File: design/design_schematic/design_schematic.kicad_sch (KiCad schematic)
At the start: 157 parts, among them IC2 XC9148G50CER-G, IC3 nRF52833-QDAA-R7, IC4 74AHCT125PW,118, IC5 MCP23018T-E_SS, IC6 XC9291B33D1R-G, J1 USB_C_Receptacle_USB2.0_16P, J2 Battery Pos, J3 Battery Neg, J4 OLED_128x32, J5 0781271220, J6 Conn_01x04, U2 BQ24072RGT, U3 USB6B1, U4 BQ27441-G1, U5 PEC11L-4015F-S0015, U6 PEC11L-4015F-S0015, X1 32MHz

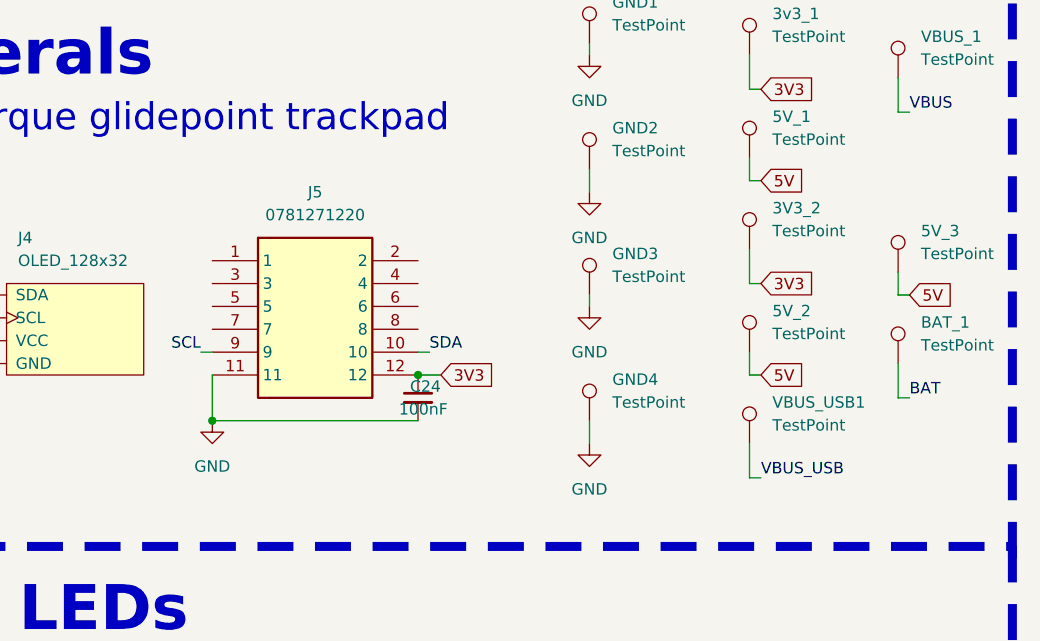
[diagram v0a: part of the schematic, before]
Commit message: routed no errors
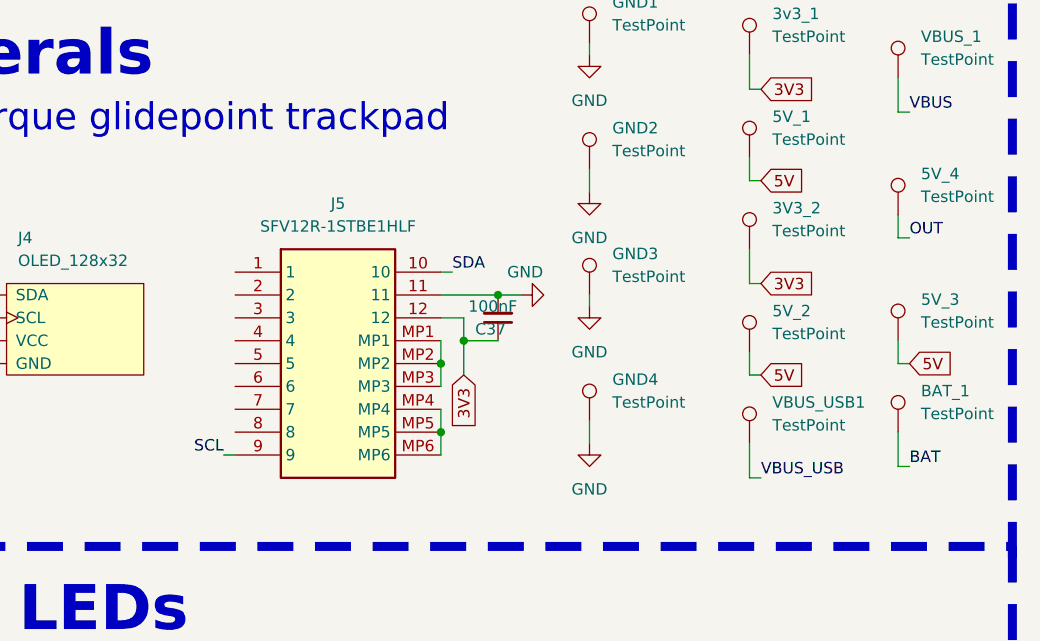
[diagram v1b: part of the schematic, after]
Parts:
- removed C24: 100nF, ScottoKeebs_Components:Capacitor_0603, symbol Device:C_Small
- removed J5: 0781271220, SamacSys_Parts:0781271220, symbol SamacSys_Parts:0781271220
- added 5V_4: TestPoint, TestPoint:TestPoint_Pad_D1.5mm, symbol Connector:TestPoint
- added C37: 100nF, ScottoKeebs_Components:Capacitor_0603, symbol Device:C_Small
- added J5: SFV12R-1STBE1HLF, SFV12R1STBE1HLF, symbol SamacSys_Parts:SFV12R-1STBE1HLF
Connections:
- net 3V3: now also C37.1, J5.12
- net GND: now also C37.2, J5.11
- net OUT: now also 5V_4.1
- net SCL: now also J5.9
- net SDA: now also J5.10
- new net: J5.MP1, J5.MP2, J5.MP3
- new net: J5.MP4, J5.MP5, J5.MP6
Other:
- moved on the sheet: 5V_3, BAT_1
